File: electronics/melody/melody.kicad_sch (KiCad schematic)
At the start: 49 parts, among them J1 USB_B, J2 Raspberry_Pi_4, J3 Conn_01x05_Pin, J4 Conn_01x01_Pin, J5 Conn_01x08_Pin, J6 Conn_01x08_Pin, J7 Conn_01x08_Pin, J8 Conn_01x08_Pin, SW1 SW_Push, SW2 SW_Push, SW3 SW_Push, SW4 SW_Push, SW5 SW_Push, SW6 SW_Push, SW7 SW_Push, U1 CD4067, U2 CD4067

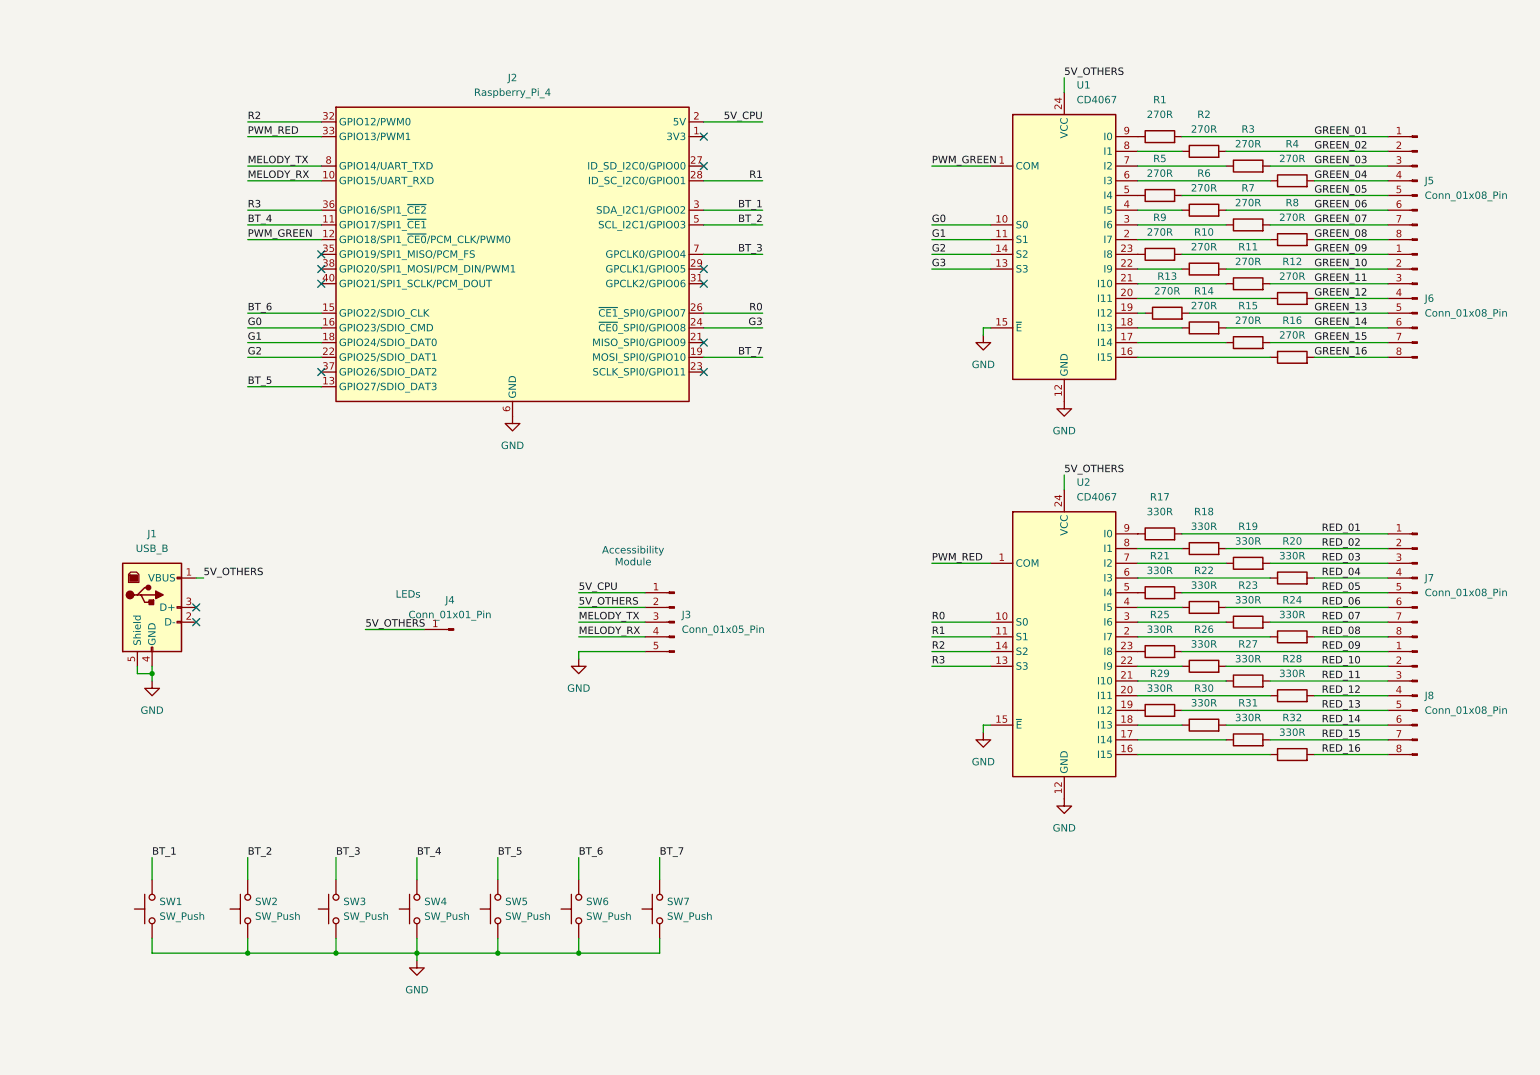
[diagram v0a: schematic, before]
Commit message: Melody schematic update
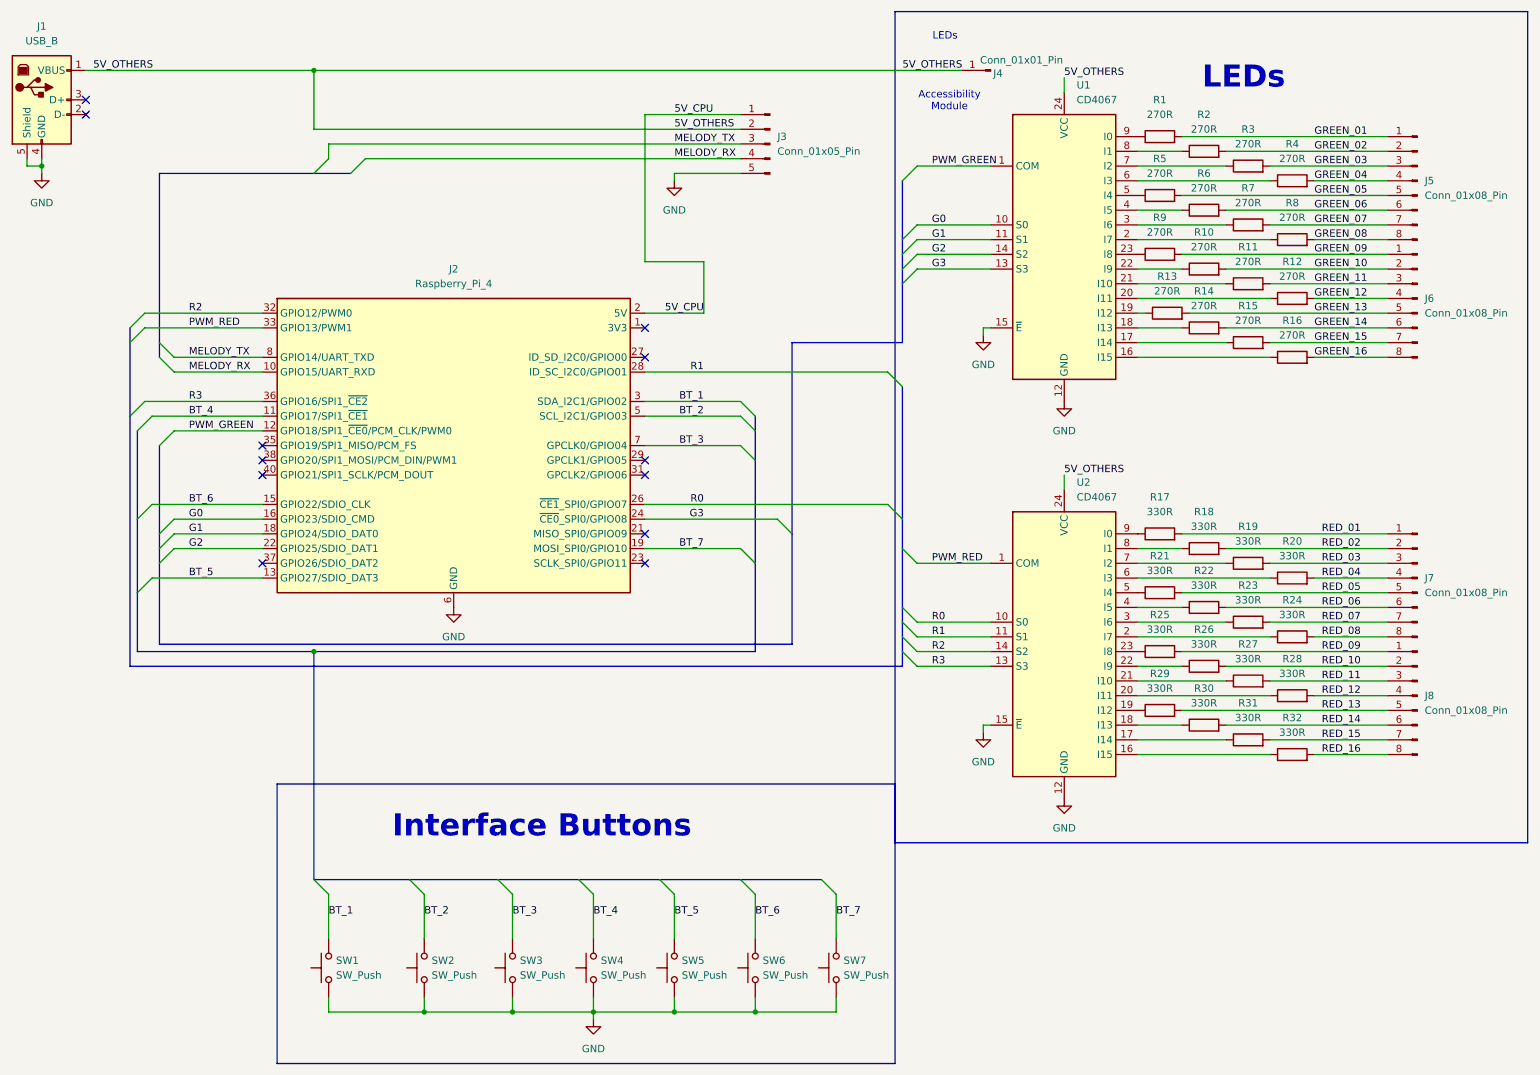
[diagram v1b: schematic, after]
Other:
- note added: "Interface Buttons"
- moved on the sheet: J1, J2, J3, J4, SW1, SW2, SW3, SW4, SW5, SW6, SW7
